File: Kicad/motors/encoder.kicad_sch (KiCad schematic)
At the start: 12 parts

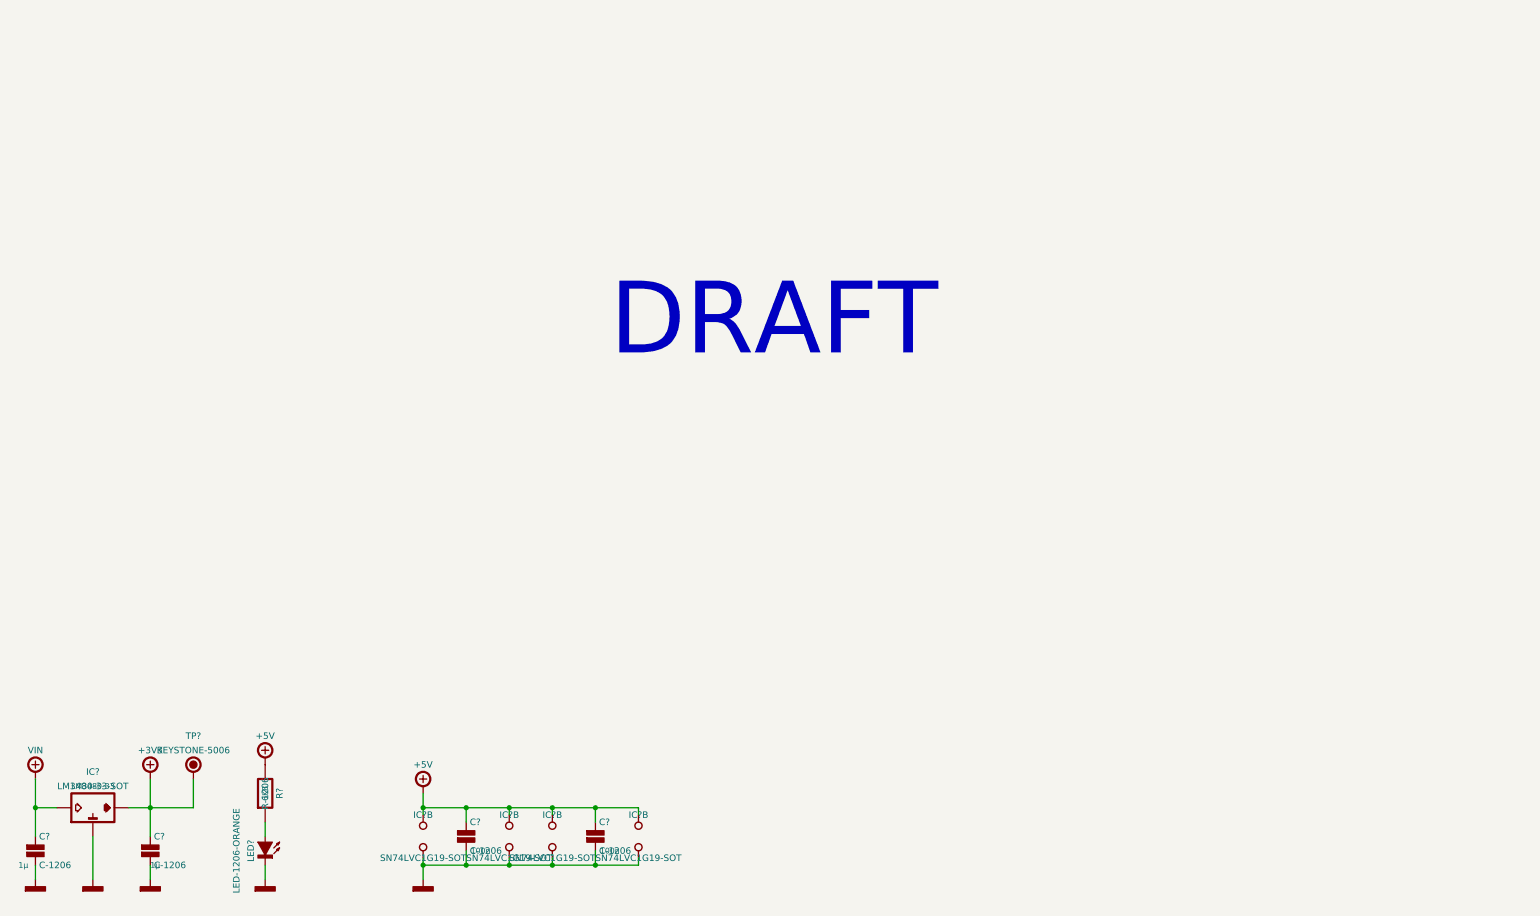
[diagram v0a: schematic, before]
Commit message: Update Motor
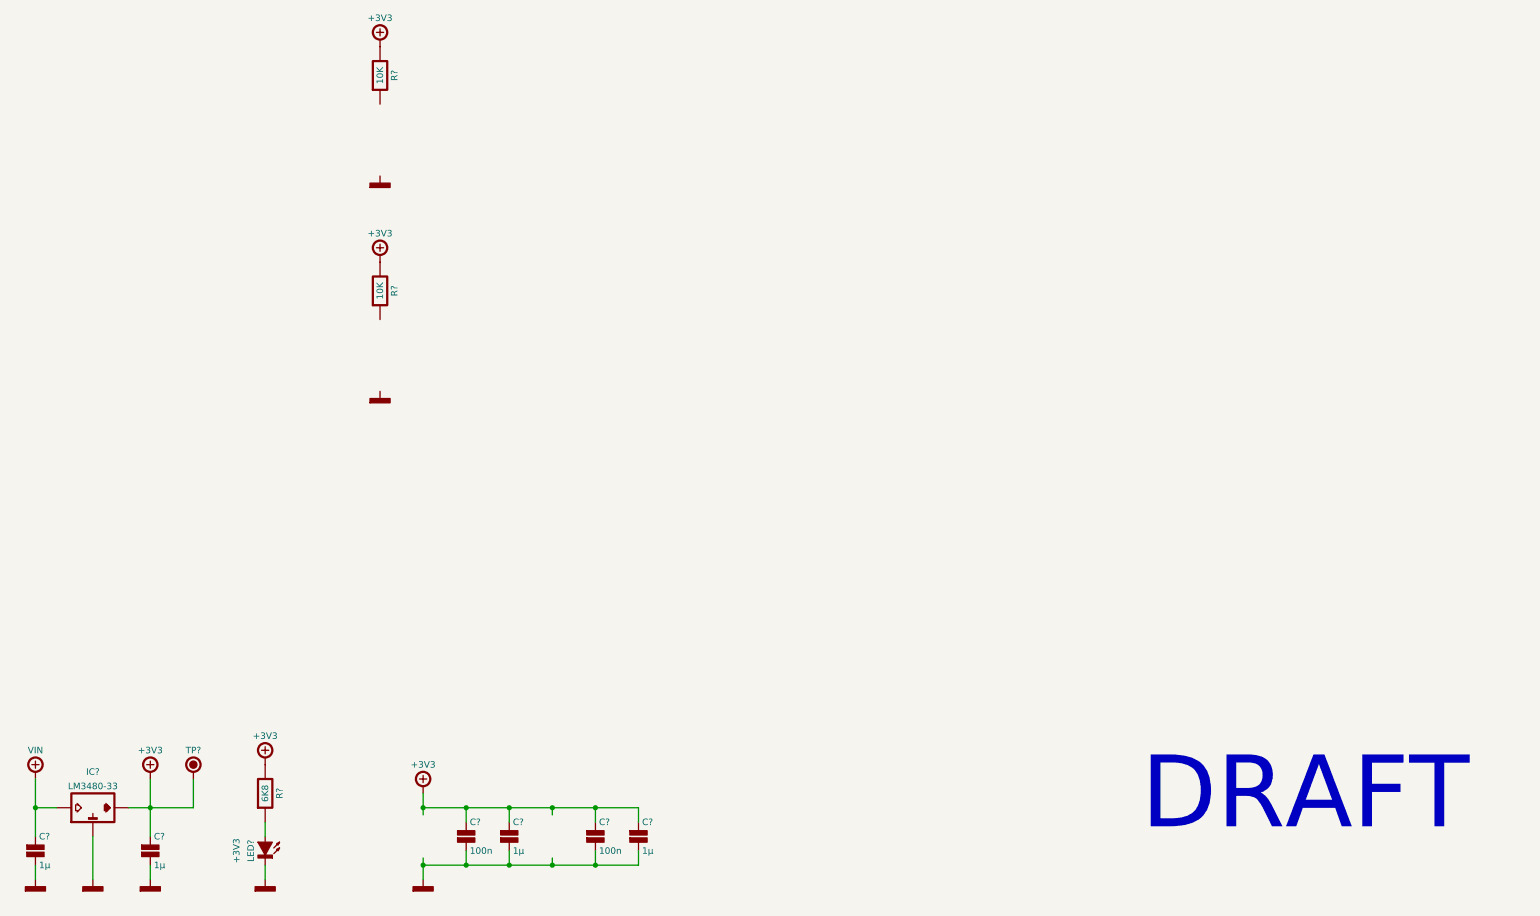
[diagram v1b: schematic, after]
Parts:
- removed IC? (x4): SN74LVC1G19-SOT, tronixio:SOT-23-6, symbol tronixio:SN74LVC1G19-SOT
- removed TP?: KEYSTONE-5006, tronixio:KEYSTONE-5006, symbol tronixio:KEYSTONE-5006
- added C? (x2): 1µ, tronixio:CAPACITOR-1206, symbol tronixio:C-1206
- added R? (x2): 10K, tronixio:RESISTOR-1206, symbol tronixio:R-1206
- added TP?: HARWIN-S1751, tronixio:zzzHARWIN-S1751, symbol tronixio:HARWIN-S1751
- C? (x2): value C-1206 -> 100n; Name 100n -> (none)
- C? (x2): value C-1206 -> 1µ; Name 1µ -> (none)
- IC?: value LM3480-33-SOT -> LM3480-33; Name LM3480-33 -> (none)
- LED?: value LED-1206-ORANGE -> +3V3; symbol tronixio:LED-1206-ORANGE -> tronixio:LED-1206-RED; MOUSER 604-APT3216LSECKJ4RV -> 604-APT3216LSECKJ3RV
- R?: value R-1206 -> 6K8; Name 6K8 -> (none)
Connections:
- net +5V is gone; now on net +3V3: C?.1, C?.1, R?.1
- net +3V3: now also C?.1, C?.1, R?.1, R?.1, TP?.1
- net GND: now also C?.2, C?.2
